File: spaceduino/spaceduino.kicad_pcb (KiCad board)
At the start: 2 copper layers, 69 x 69 mm, 87 parts, among them J1 USB_B, J2 Micro_SD_Card, J3 JICSP, J4 Conn_02x05_Odd_Even, Q1 BSS84, Q2 BSS84, Q3 BSS84, Q4 BC856BS, Q5 BSS84, SW1 SW_SPST, U1 TLV70030_SOT23-5, U2 FT230XS, U3 TXB0104D, U4 LM27313XMF, U5 INA226, U6 ATmega1284P-AU, U7 INA226, U8 MPD200A, U9 INA226, Y1 Crystal

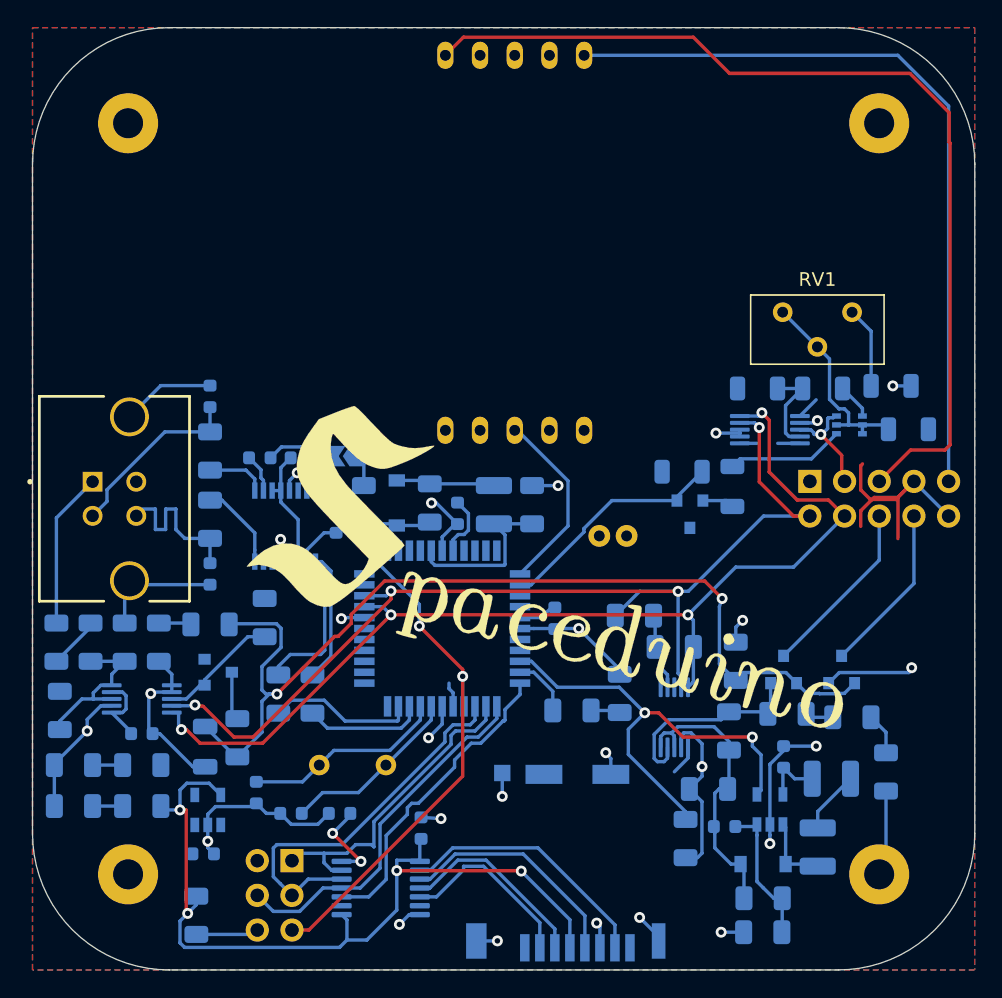
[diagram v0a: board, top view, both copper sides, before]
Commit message: can i get a go dawgs
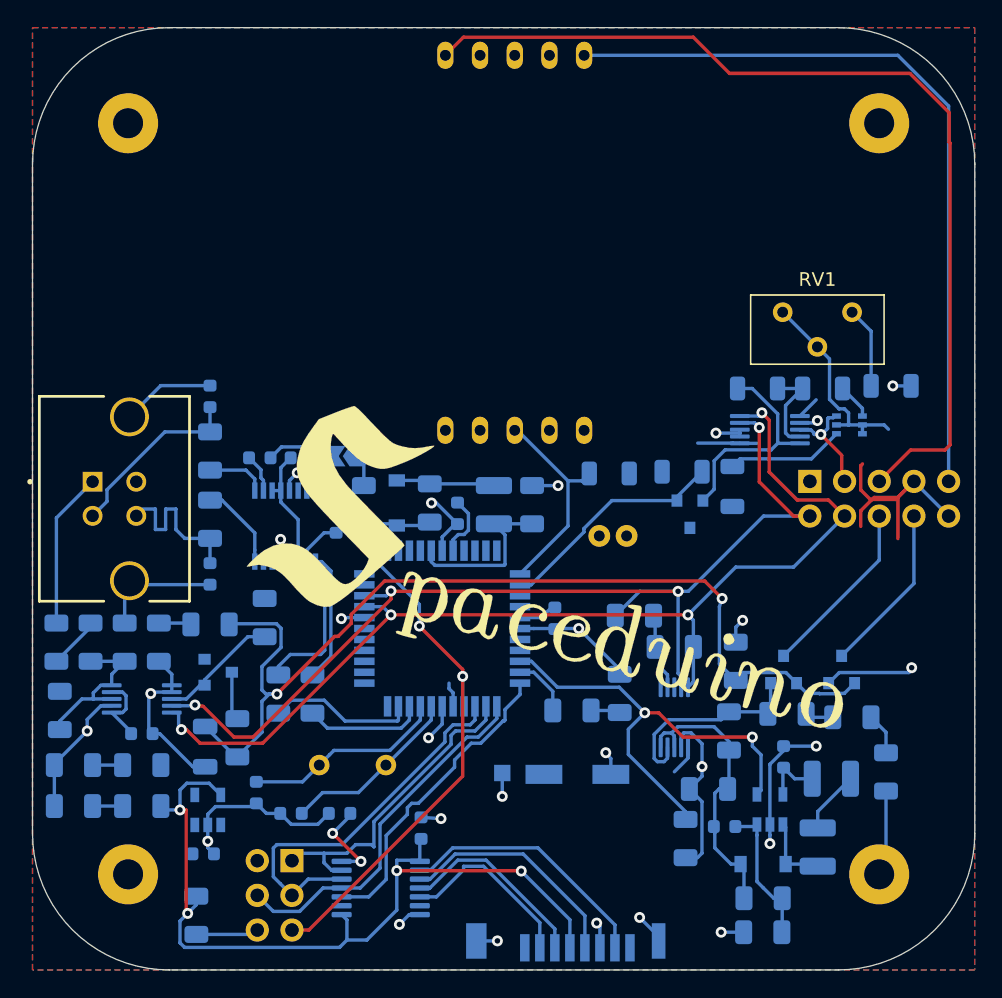
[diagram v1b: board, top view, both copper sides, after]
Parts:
- moved R26 22.1 mm to (98.2, 88.6)
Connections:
- R22 pad 1: +5V -> Net-(Q5-Pad2)
- R23 pad 1: Net-(Q5-Pad2) -> +5V
- R26 pad 2: Net-(Q4-Pad2) -> a3_pump_en
- U9 pad 10: +5V -> Net-(Q5-Pad2)
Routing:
- net Net-(Q5-Pad2): track 2.34 -> 15.9 mm
- net a3_pump_en: track 13.7 -> 15.5 mm
- net +5V: track 55.5 -> 57.0 mm
